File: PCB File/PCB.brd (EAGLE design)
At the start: 53.4 x 96.1 mm, 12 parts

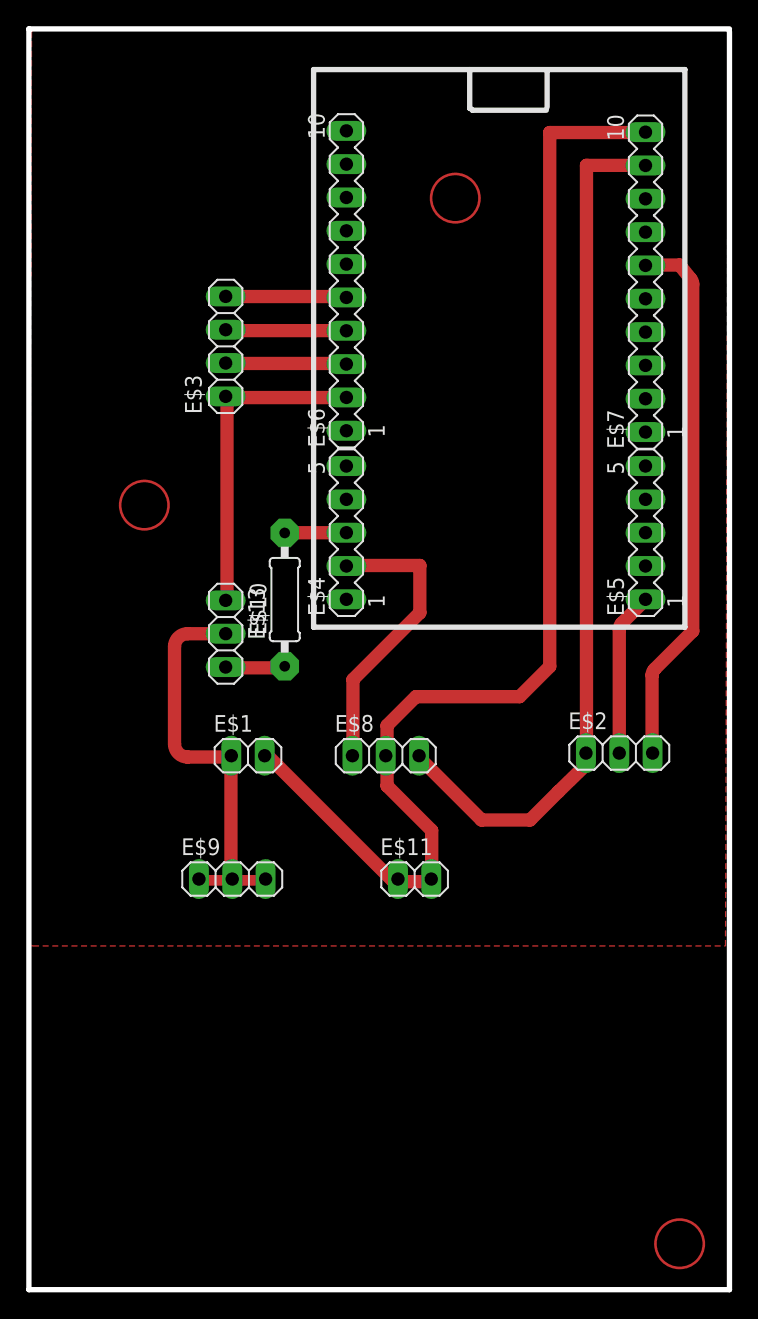
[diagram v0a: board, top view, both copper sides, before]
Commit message: Sync
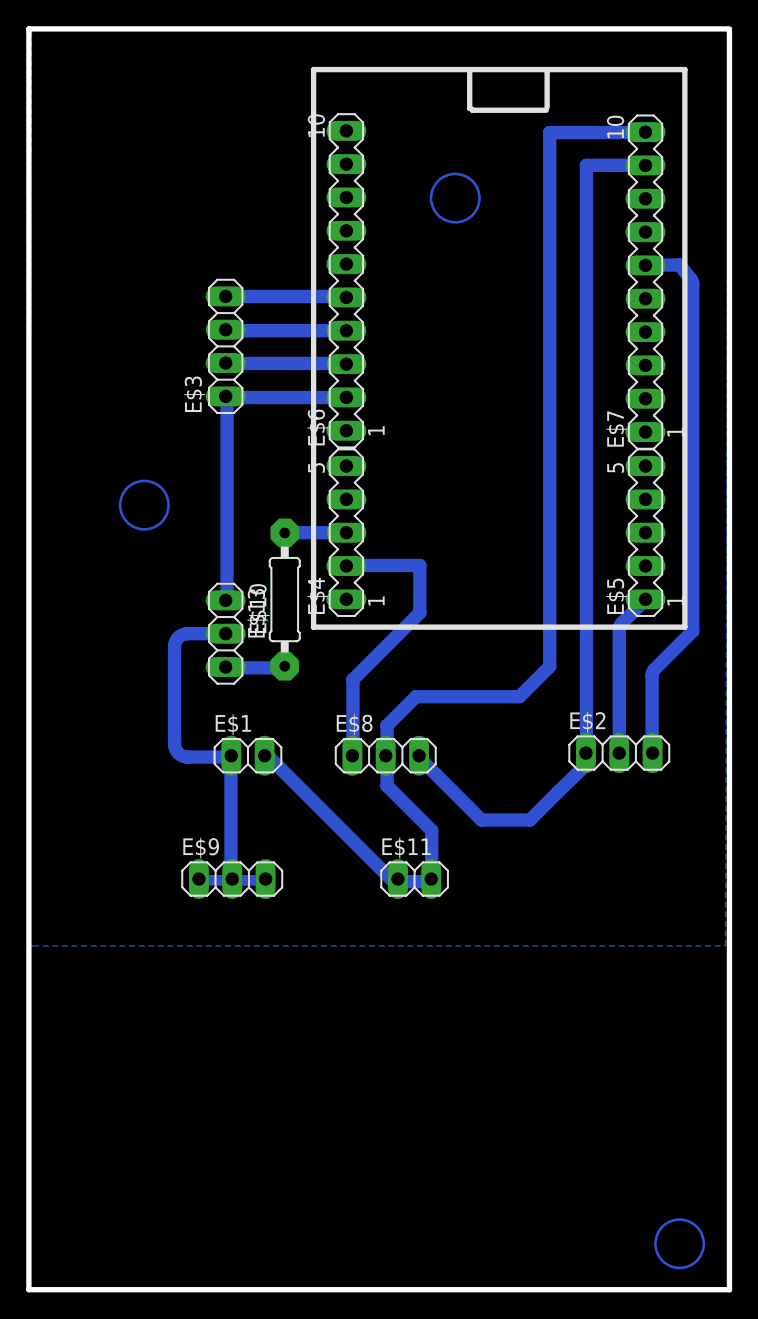
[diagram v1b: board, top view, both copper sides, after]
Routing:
- net 5VDC: track 92.6 -> 92.5 mm, vias 0 -> 1
- added copper zone on layer 16, net GND
- removed copper zone on layer 1, net GND
